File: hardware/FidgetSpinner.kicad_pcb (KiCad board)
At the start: 2 copper layers, 71.9 x 65.7 mm, 25 parts, among them J1 ICSP, J2 ICSP, SW1 ON/OFF, U1 ATmega328P-A, U2 L78L05, Y1 16Mhz

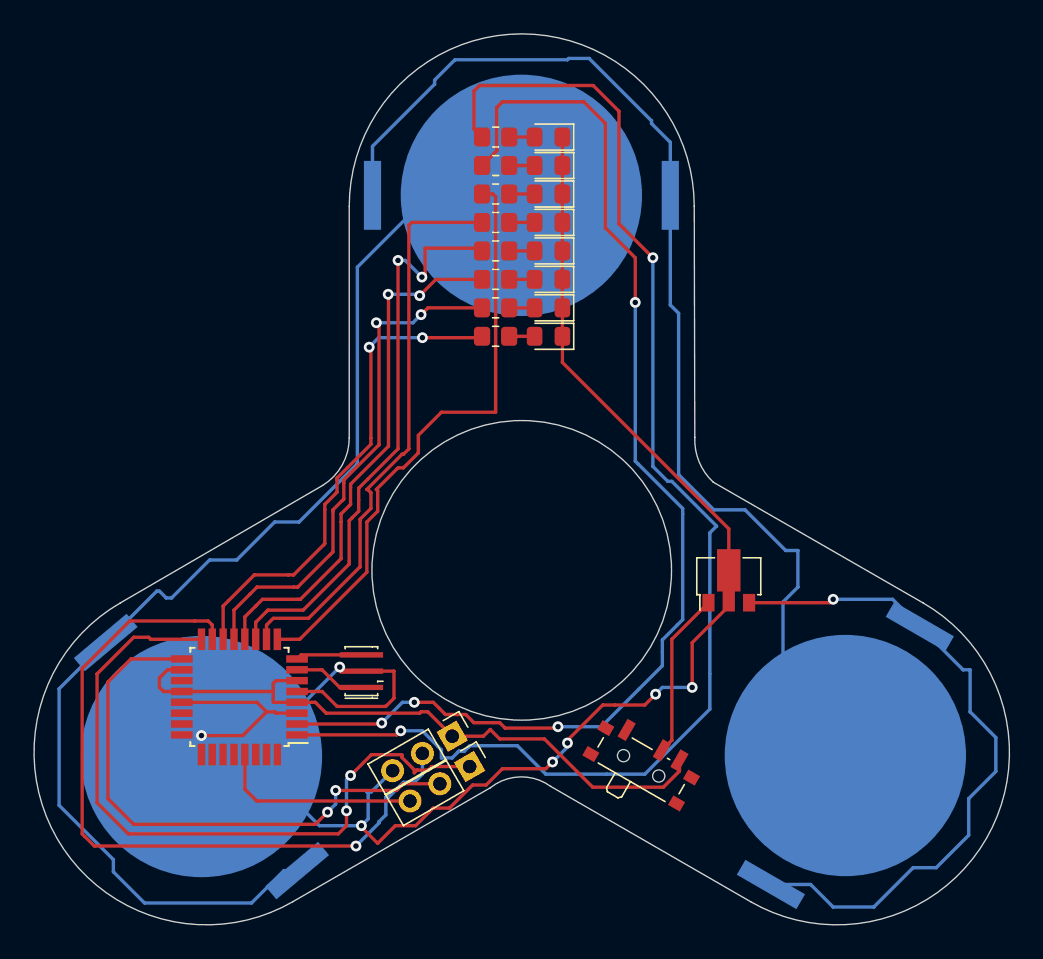
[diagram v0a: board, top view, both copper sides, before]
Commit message: update code
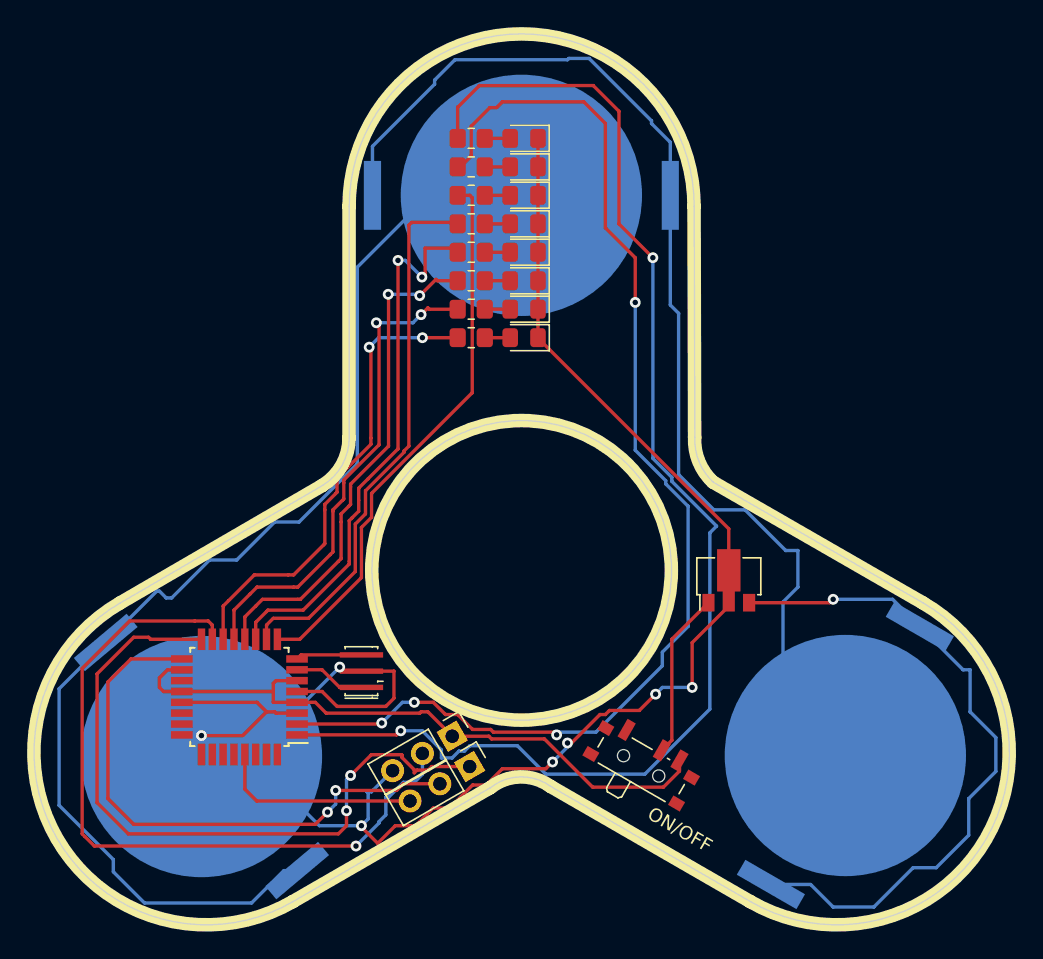
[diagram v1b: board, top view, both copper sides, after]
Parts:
- moved D1 1.80 mm to (158.1, 69.2)
- moved D3 1.80 mm to (158.1, 73.4)
- moved D6 1.80 mm to (158.1, 79.7)
- moved D8 1.80 mm to (158.1, 83.9)
- moved R1 1.80 mm to (154.2, 69.2)
- moved R3 1.80 mm to (154.2, 73.4)
- moved R6 1.80 mm to (154.2, 79.7)
- moved R8 1.80 mm to (154.2, 83.9)
- moved D2 1.80 mm to (158.1, 71.3)
- moved D4 1.80 mm to (158.1, 75.5)
- moved D5 1.80 mm to (158.1, 77.6)
- moved D7 1.80 mm to (158.1, 81.8)
- moved R2 1.80 mm to (154.2, 71.3)
- moved R4 1.80 mm to (154.2, 75.5)
- moved R5 1.80 mm to (154.2, 77.6)
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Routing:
- net LED3: track 44.0 -> 40.6 mm
- net LED4: track 42.2 -> 40.1 mm
- net LED2: track 86.9 -> 88.9 mm
- net LED8: track 36.5 -> 34.6 mm
- net LED5: track 42.6 -> 40.8 mm
- net LED7: track 37.9 -> 36.1 mm
- net LED6: track 39.0 -> 37.2 mm
- net GND: track 133.7 -> 134.3 mm
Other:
- board text added: "5V"
- board text added: "GND"
- board text added: "MISO"
- board text added: "MOSI"
- board text added: "RST"
- board text added: "SCK"
- board text added: "https://github.com/zosko/FidgetSpinner by Bosko"
